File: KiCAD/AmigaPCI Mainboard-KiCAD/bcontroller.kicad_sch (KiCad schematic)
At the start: 20 parts, among them CN227 JTAG/SWD, J200 DISABLE AUTOBOOT, U6 XC95144XL-TQ144, U711 XC9572XL-VQ64

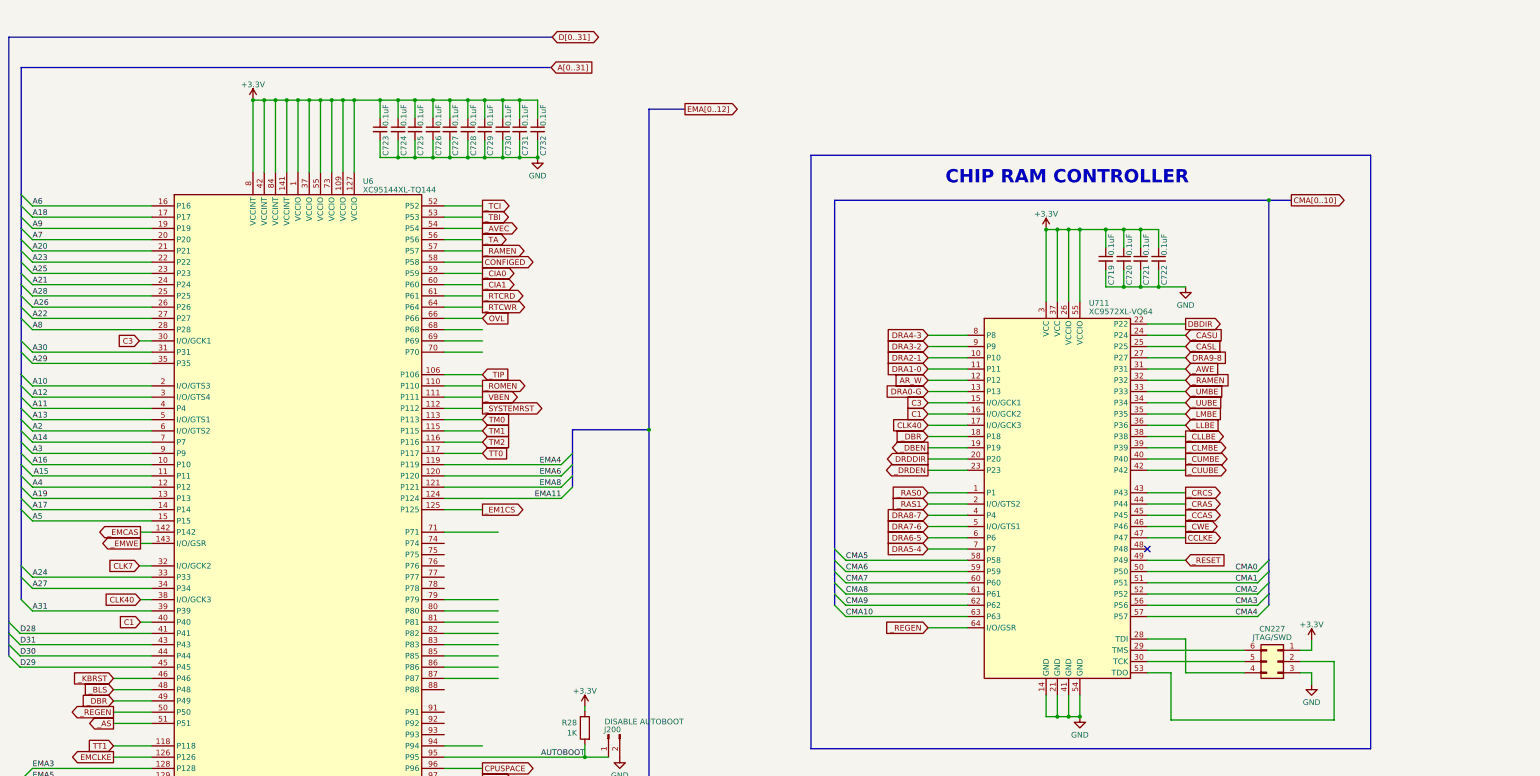
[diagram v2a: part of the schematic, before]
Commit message: Routing 19-DEC-2023
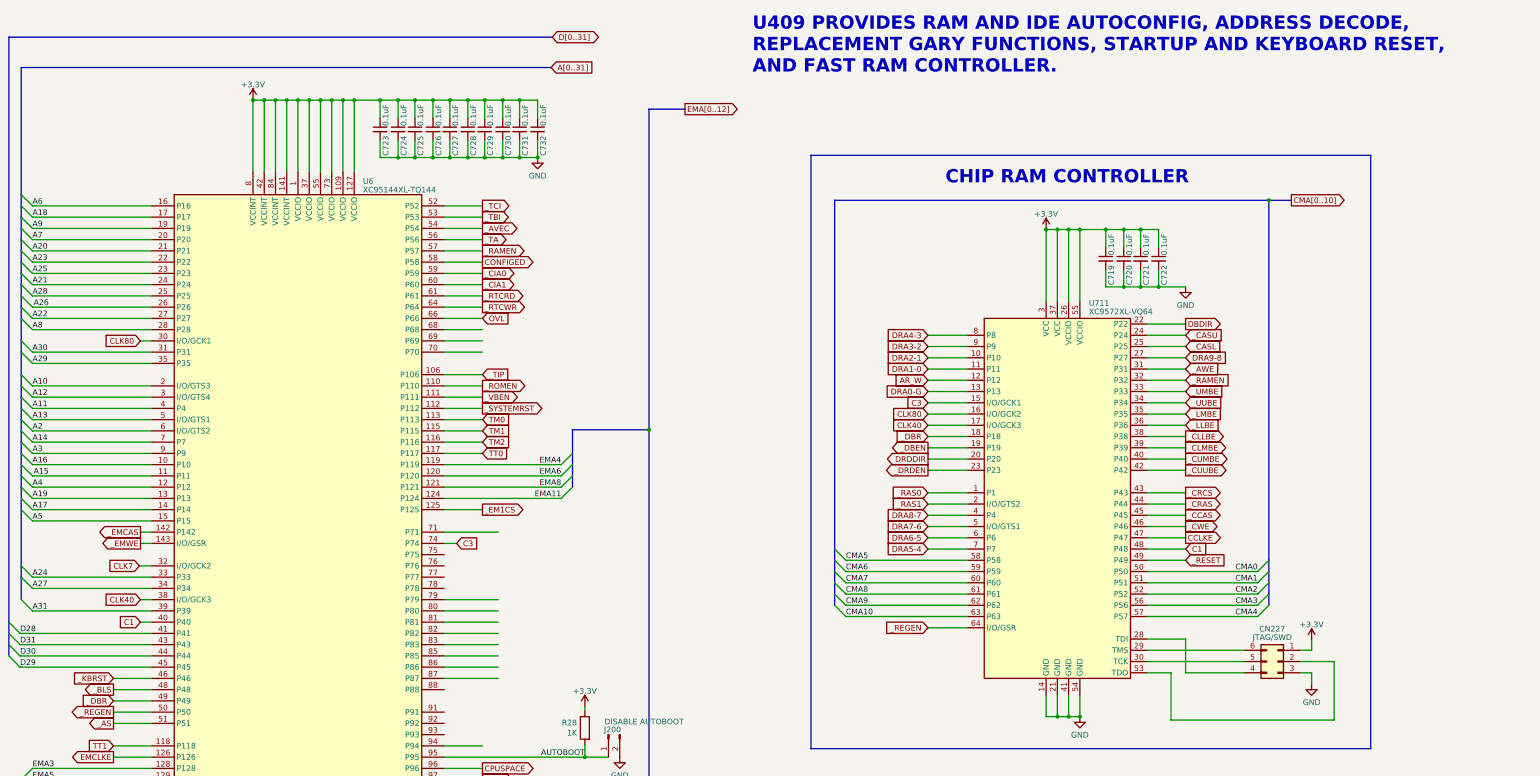
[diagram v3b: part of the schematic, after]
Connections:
- net C1: now also U711.48 (P48); no longer U711.16 (I/O/GCK2)
- net C3: now also U6.74 (P74); no longer U6.30 (I/O/GCK1)
- new net CLK80: U6.30 (I/O/GCK1), U711.16 (I/O/GCK2)
- no-connect marks 1 -> 0
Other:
- note added: "U409 PROVIDES RAM AND IDE AUTOCONFIG, ADDRESS DECODE, REPLACEMENT GARY FUNCTIONS, STARTUP AND KEYBOARD RESET, AND FAST RAM CONTROLLER."
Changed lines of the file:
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@@
   (junction (at 192.024 59.69) (diameter 0) (color 0 0 0 0)
   )
-  (no_connect (at 337.566 148.082))
   (bus_entry (at 85.852 134.112) (size -2.54 -2.54)
     (stroke (width 0) (type default))
@@
     (stroke (width 0) (type default))
   )
-  (wire (pts (xy 109.982 101.092) (xy 112.776 101.092))
+  (wire (pts (xy 181.61 146.812) (xy 178.816 146.812))
     (stroke (width 0) (type default))
   )
@@
     (stroke (width 0) (type default))
   )
+  (wire (pts (xy 110.236 101.092) (xy 112.776 101.092))
+    (stroke (width 0) (type default))
+  )
   (bus (pts (xy 83.312 136.906) (xy 83.312 139.192))
     (stroke (width 0) (type default))
@@
     (stroke (width 0) (type default))
   )
+  (wire (pts (xy 288.036 117.602) (xy 296.926 117.602))
+    (stroke (width 0) (type default))
+  )
   (wire (pts (xy 110.236 159.512) (xy 112.776 159.512))
     (stroke (width 0) (type default))
@@
     (stroke (width 0) (type default))
   )
-  (wire (pts (xy 288.036 117.602) (xy 296.926 117.602))
+  (wire (pts (xy 346.202 148.082) (xy 337.566 148.082))
     (stroke (width 0) (type default))
   )
@@
   )
   (text "CHIP RAM CONTROLLER" (at 291.973 65.913 0)
+    (effects (font (size 3 3) (thickness 0.6) bold) (justify left bottom))
+  )
+  (text "U409 PROVIDES RAM AND IDE AUTOCONFIG, ADDRESS DECODE,\nREPLACEMENT GARY FUNCTIONS, STARTUP AND KEYBOARD RESET, \nAND FAST RAM CONTROLLER."
+    (at 248.412 40.894 0)
     (effects (font (size 3 3) (thickness 0.6) bold) (justify left bottom))
   )
@@
     )
   )
-  (global_label "C3" (shape input) (at 109.982 101.092 180) (fields_autoplaced)
-    (effects (font (size 1.27 1.27)) (justify right))
-    (property "Intersheetrefs" "${INTERSHEET_REFS}" (at 104.5967 101.092 0)
-      (effects (font (size 1.27 1.27)) (justify right))
+  (global_label "C3" (shape input) (at 181.61 146.812 0) (fields_autoplaced)
+    (effects (font (size 1.27 1.27)) (justify left))
+    (property "Intersheetrefs" "${INTERSHEET_REFS}" (at 186.9953 146.812 0)
+      (effects (font (size 1.27 1.27)) (justify left))
     )
   )
@@
     )
   )
-  (global_label "C1" (shape input) (at 288.036 117.602 180) (fields_autoplaced)
+  (global_label "C1" (shape input) (at 346.202 148.082 0) (fields_autoplaced)
+    (effects (font (size 1.27 1.27)) (justify left))
+    (property "Intersheetrefs" "${INTERSHEET_REFS}" (at 351.6667 148.082 0)
+      (effects (font (size 1.27 1.27)) (justify left))
+    )
+  )
+  (global_label "_CUMBE" (shape output) (at 346.202 127.762 0) (fields_autoplaced)
+    (effects (font (size 1.27 1.27)) (justify left))
+    (property "Intersheetrefs" "${INTERSHEET_REFS}" (at 356.5463 127.762 0)
+      (effects (font (size 1.27 1.27)) (justify left))
+    )
+  )
+  (global_label "CLK80" (shape input) (at 288.036 117.602 180) (fields_autoplaced)
     (effects (font (size 1.27 1.27)) (justify right))
-    (property "Intersheetrefs" "${INTERSHEET_REFS}" (at 282.6507 117.602 0)
-      (effects (font (size 1.27 1.27)) (justify right))
-    )
-  )
-  (global_label "_CUMBE" (shape output) (at 346.202 127.762 0) (fields_autoplaced)
-    (effects (font (size 1.27 1.27)) (justify left))
-    (property "Intersheetrefs" "${INTERSHEET_REFS}" (at 356.5463 127.762 0)
-      (effects (font (size 1.27 1.27)) (justify left))
+    (property "Intersheetrefs" "${INTERSHEET_REFS}" (at 279.0637 117.602 0)
+      (effects (font (size 1.27 1.27)) (justify right))
     )
   )
@@
     )
   )
+  (global_label "CLK80" (shape input) (at 110.236 101.092 180) (fields_autoplaced)
+    (effects (font (size 1.27 1.27)) (justify right))
+    (property "Intersheetrefs" "${INTERSHEET_REFS}" (at 101.2637 101.092 0)
+      (effects (font (size 1.27 1.27)) (justify right))
+    )
+  )
   (global_label "_AS" (shape output) (at 104.14 187.452 180) (fields_autoplaced)
     (effects (font (size 1.27 1.27)) (justify right))
@@
     )
   )
-  (global_label "_BLS" (shape input) (at 104.14 179.832 180) (fields_autoplaced)
+  (global_label "_BLS" (shape output) (at 104.14 179.832 180) (fields_autoplaced)
     (effects (font (size 1.27 1.27)) (justify right))
     (property "Intersheetrefs" "${INTERSHEET_REFS}" (at 96.6796 179.832 0)
